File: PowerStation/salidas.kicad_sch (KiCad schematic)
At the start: 7 parts, among them J1 Salidas, SW1 SW_Push_Dual, SW2 SW_Push_Dual

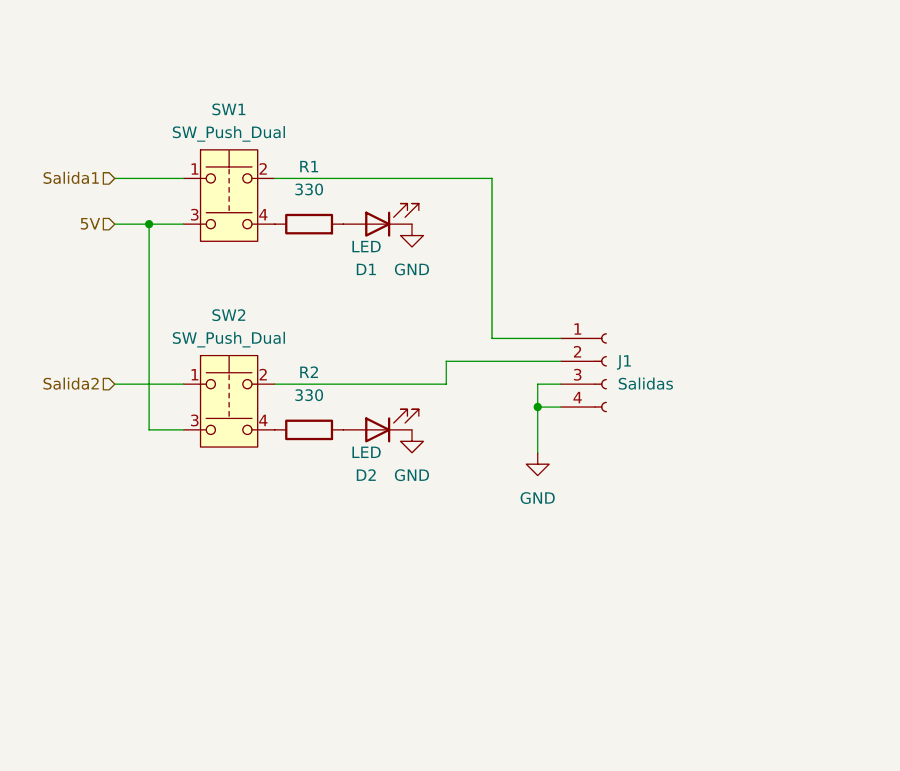
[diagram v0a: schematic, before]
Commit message: correccion de esquermatico y avanze en placa
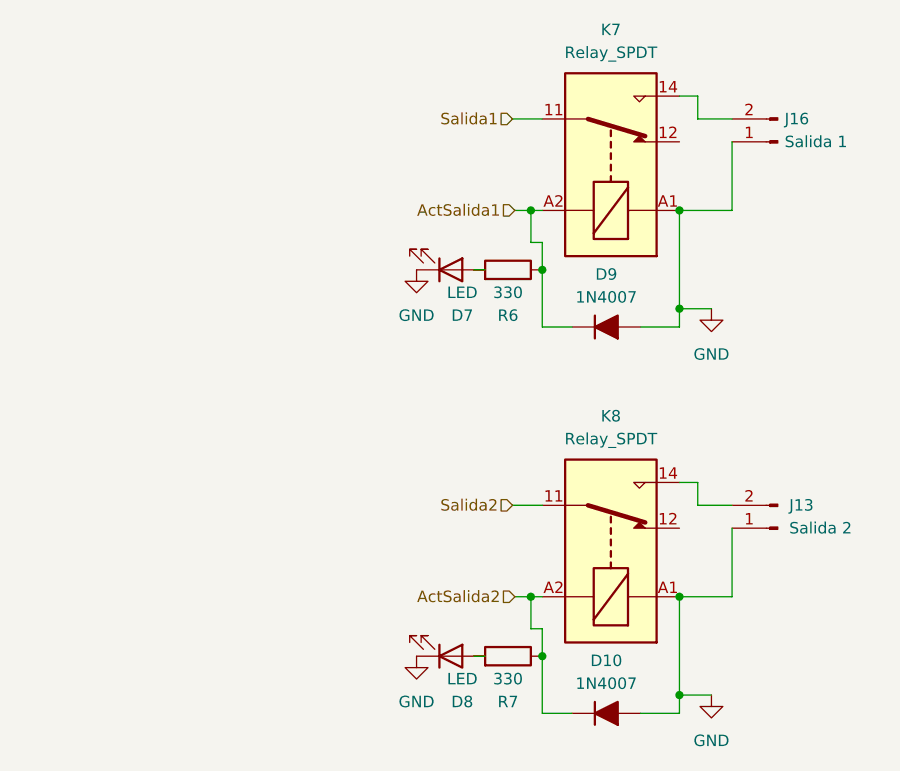
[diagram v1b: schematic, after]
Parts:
- removed D2: LED, LED_SMD:LED_0805_2012Metric, symbol Device:LED
- removed J1: Salidas, Connector_JST:JST_NV_B04P-NV_1x04_P5.00mm_Vertical, symbol Connector:Conn_01x04_Socket
- removed R2: 330, Resistor_SMD:R_0402_1005Metric, symbol Device:R
- removed SW1, SW2: SW_Push_Dual, Connector:FanPinHeader_1x04_P2.54mm_Vertical, symbol Switch:SW_Push_Dual
- added D10, D9: 1N4007, Diode_SMD:D_SMA, symbol PCM_Diode_AKL:1N4007
- added D8: LED, LED_SMD:LED_0805_2012Metric, symbol Device:LED
- added J13: Salida 2, Connector:JWT_A3963_1x02_P3.96mm_Vertical, symbol Connector:Conn_01x02_Pin
- added J16: Salida 1, Connector:JWT_A3963_1x02_P3.96mm_Vertical, symbol Connector:Conn_01x02_Pin
- added K7, K8: Relay_SPDT, Relay_THT:Relay_SPDT_Finder_36.11, symbol Relay:Relay_SPDT
- added R7: 330, Resistor_SMD:R_0402_1005Metric, symbol Device:R
- renumbered D1 to D7, R1 to R6
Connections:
- net GND: now also D10.2 (A), D8.1 (K), D9.2 (A), J13.1 (Pin_1), J16.1 (Pin_1), K7.A1, K8.A1
- net Salida1: now also K7.11
- net Salida2: now also K8.11
- net ActSalida1: now reaches R6.1
- net ActSalida1: now also D9.1 (K), K7.A2
- new net: J13.2 (Pin_2), K8.14
- new net: D8.2 (A), R7.2
- new net: J16.2 (Pin_2), K7.14
- new net ActSalida2: D10.1 (K), K8.A2, R7.1
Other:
- moved on the sheet: D7, R6
